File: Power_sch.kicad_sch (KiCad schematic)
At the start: 47 parts, among them J1 USB4105-GF-A, J2 USB4105-GF-A, U2 TPD2EUSB30ADRTR, U6 ADP150WACBZ-3.3-R7, U7 IR3883MTRPBF, U9 LM66200DRLR

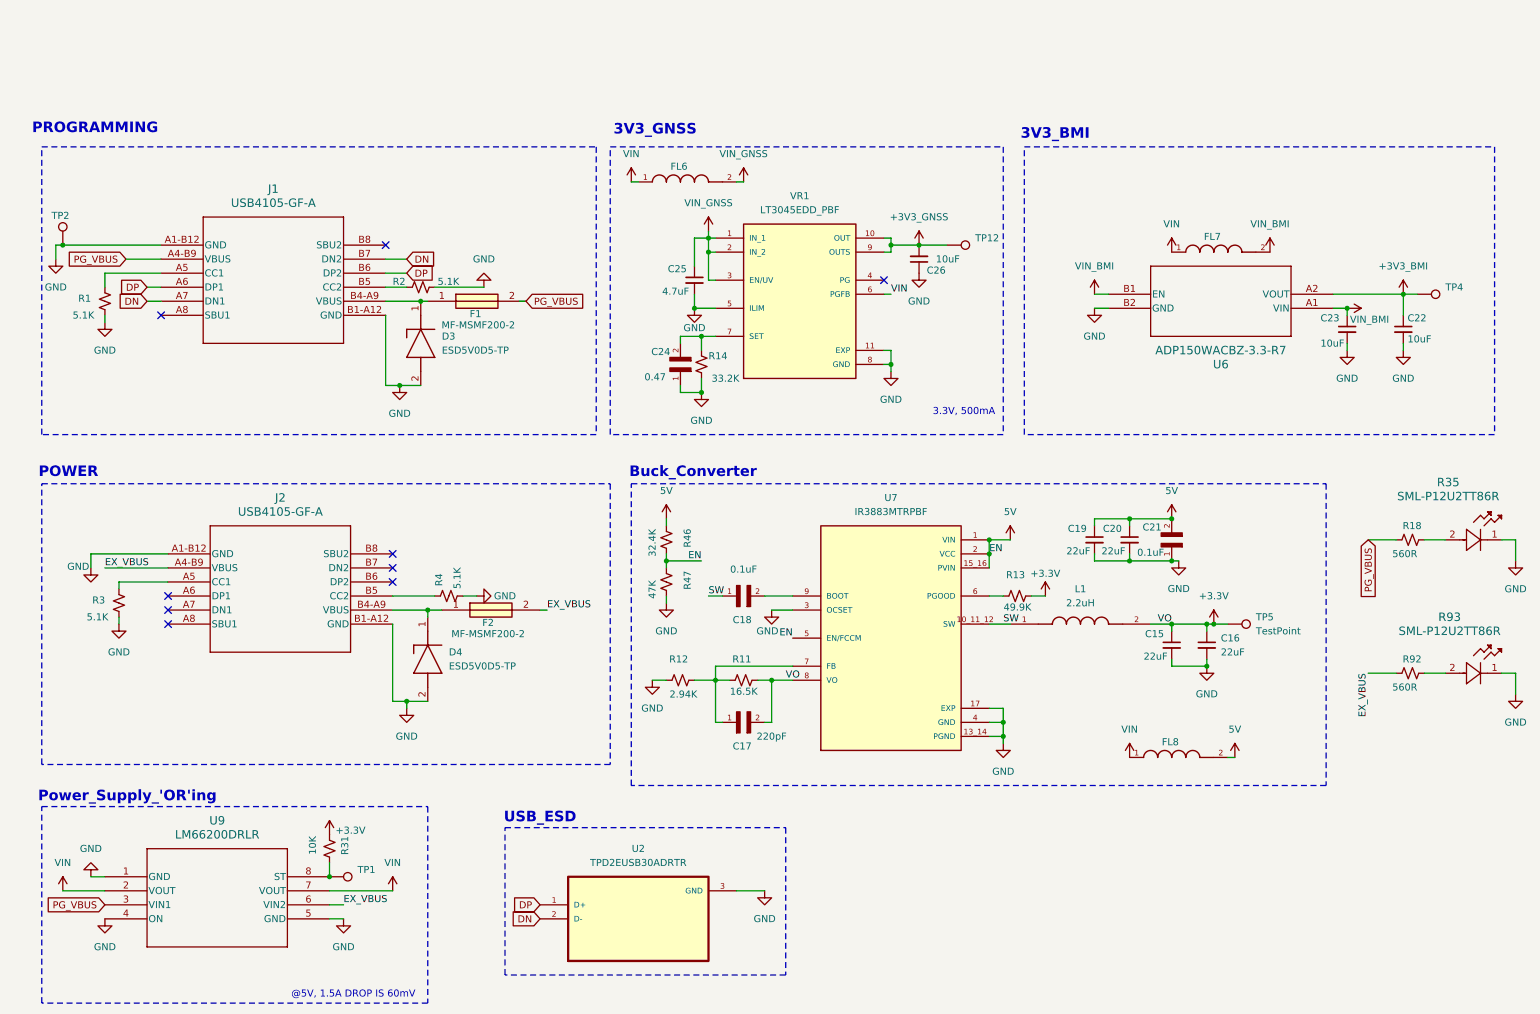
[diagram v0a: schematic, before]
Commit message: new
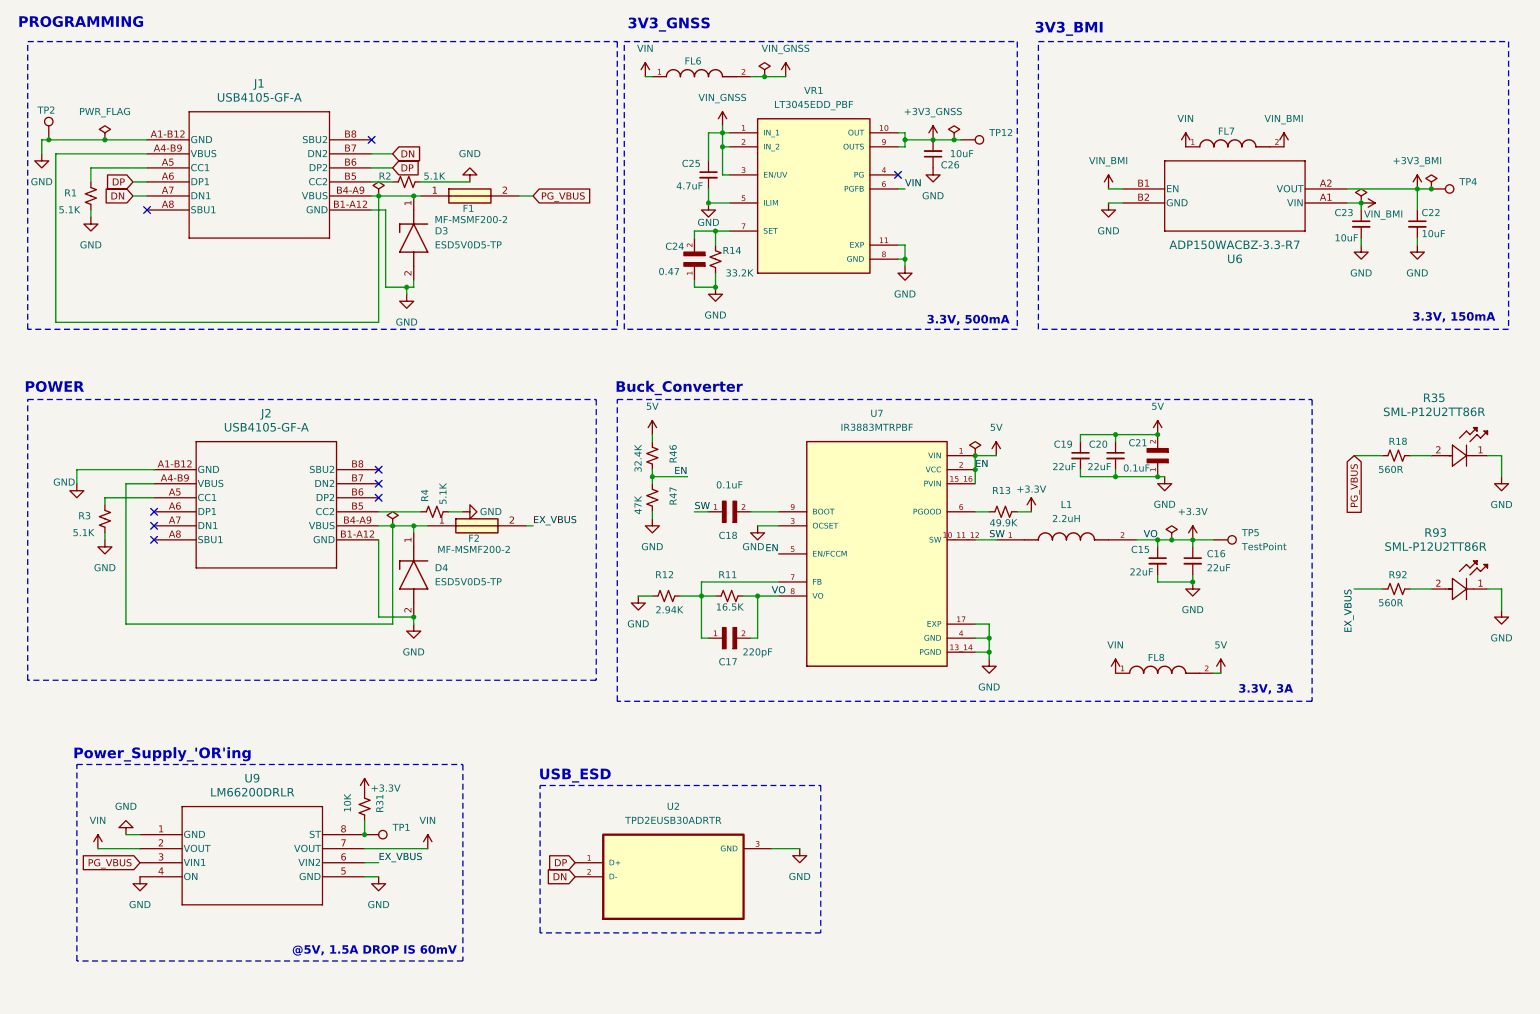
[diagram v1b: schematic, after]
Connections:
- net EX_VBUS: no longer J2.A4-B9 (VBUS)
- net PG_VBUS: no longer J1.A4-B9 (VBUS)
- net at D4.1 (K), F2.1, J2.B4-A9 (VBUS): now also J2.A4-B9 (VBUS)
- net at D3.1 (K), F1.1, J1.B4-A9 (VBUS): now also J1.A4-B9 (VBUS)
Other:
- note added: "3.3V, 150mA"
- note added: "3.3V, 3A"
- moved on the sheet: C15, C16, C17, C18, C19, C20, C21, C22, C23, C24, C25, C26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

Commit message: schematics
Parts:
- D4: footprint ESD5V0D5TP -> GNSS:ESD5V0D5TP
- F1, F2: footprint FUSC4632X85N -> GNSS:FUSC4632X85N
- U2: footprint (none) -> GNSS:SOTFL35P100X50-3N
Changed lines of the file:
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@@
 			)
 		)
-		(property "Footprint" "FUSC4632X85N"
+		(property "Footprint" "GNSS:FUSC4632X85N"
 			(at 100.33 202.87 0)
 			(effects
@@
 			)
 		)
-		(property "Footprint" ""
+		(property "Footprint" "GNSS:SOTFL35P100X50-3N"
 			(at 130.81 170.18 0)
 			(effects
@@
 			)
 		)
-		(property "Footprint" "FUSC4632X85N"
+		(property "Footprint" "GNSS:FUSC4632X85N"
 			(at 99.06 143.18 0)
 			(effects
@@
 			)
 		)
-		(property "Footprint" "ESD5V0D5TP"
+		(property "Footprint" "GNSS:ESD5V0D5TP"
 			(at -9.83 118.11 0)
 			(effects
